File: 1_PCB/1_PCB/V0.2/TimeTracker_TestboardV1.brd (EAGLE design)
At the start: 105.1 x 80 mm, 47 parts, among them IC1 L78L33ABUTR, IC2 7805DT, IC3 PCF8574T_3,518, IC4 PCF8574T_3,518, U1 WS2812B, U2 WS2812B, U3 WS2812B, U4 WS2812B, U5 SMTM1225, Y1 FX135A-327

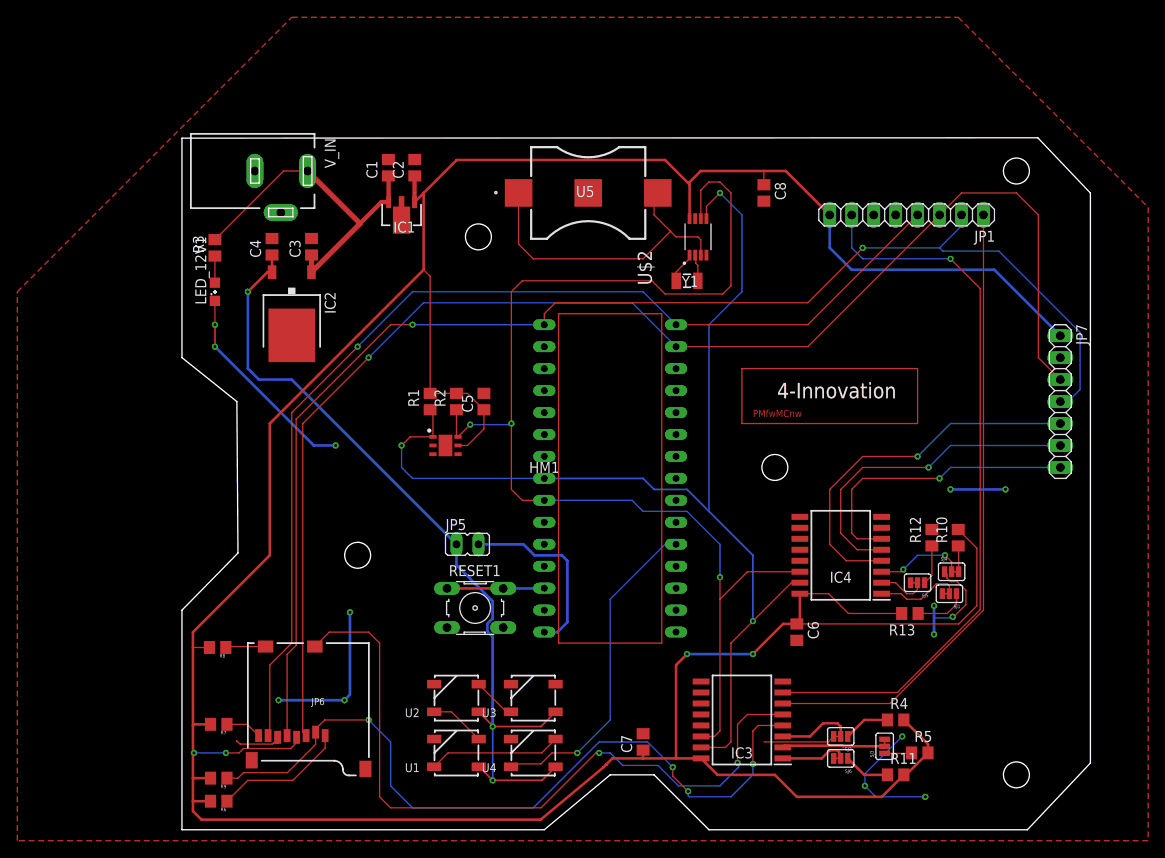
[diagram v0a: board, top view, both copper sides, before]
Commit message: Nicolas
PCB Update
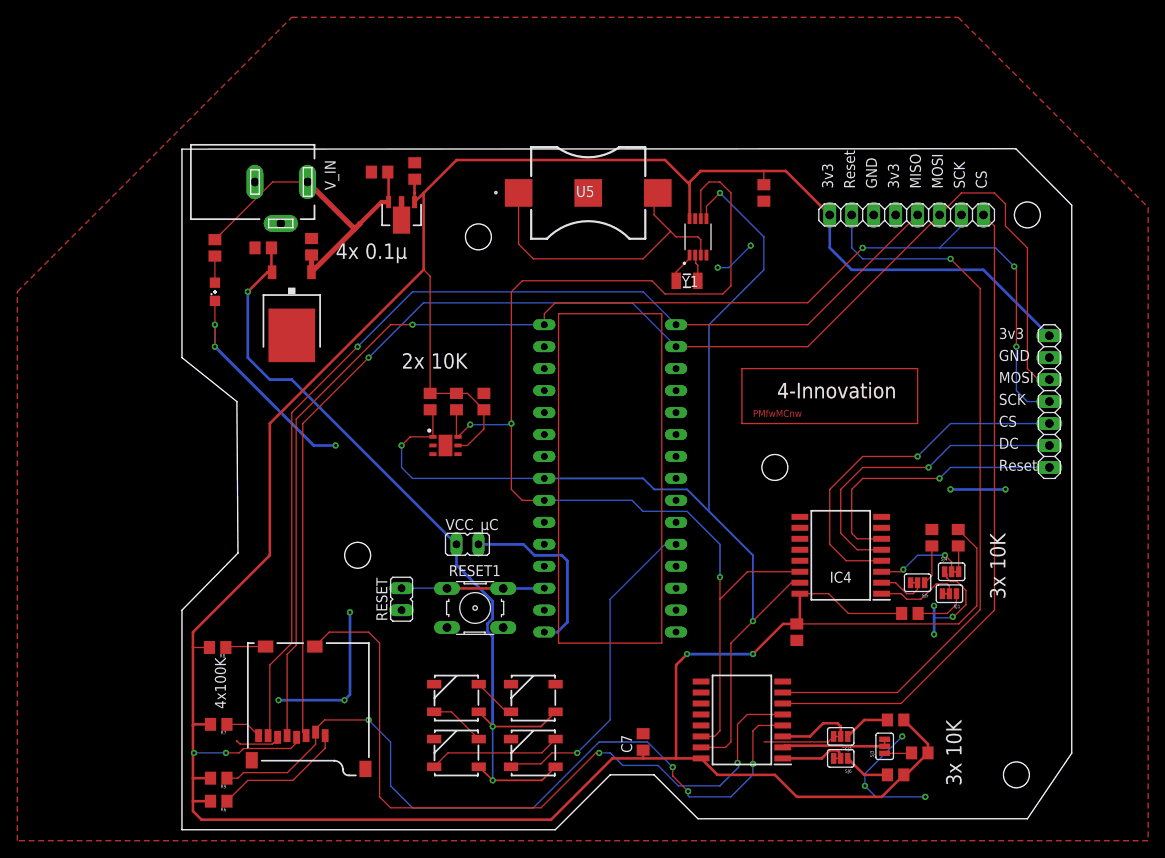
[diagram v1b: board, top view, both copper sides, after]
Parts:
- removed C1: (no value), rcl:C0805
- added 0.1µ: (no value), rcl:C0805
- added RESET: (no value), jumper:JP1
- C2, C6, C8: value (none) -> 0,1µ
- moved V_IN 1.27 mm to (8.89, 73.7)
- moved JP7 1.27 mm to (97.8, 48.3)
- moved C4 1.02 mm to (6.86, 66.0), turned to 180 degrees
- moved C2 0.38 mm to (24.4, 74.9)
- renumbered JP5 to VCC_µC
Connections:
- net GND: now also 0.1µ.2, RESET.1; no longer C1.2
- net GND1: now also RESET.2
- net N$1: now also 0.1µ.1; no longer C1.1
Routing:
- net GND1: track 11.3 -> 16.5 mm
- net GND: track 92.9 -> 97.7 mm, vias 14 -> 16
- net I2CSDA: track 131.4 -> 133.5 mm
- net RFID_CS: track 73.4 -> 75.2 mm
- net 3V3: track 401.3 -> 399.8 mm
- net SPISCK: track 155.1 -> 153.6 mm, vias 2 -> 4
- net SPIMOSI: track 157.8 -> 156.5 mm
- net DISPLAY_RESET: track 34.0 -> 32.7 mm
- net DISPLAY_DC: track 38.1 -> 36.8 mm
- net DISPLAY_CS: track 43.0 -> 41.7 mm
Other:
- board size 105.1 x 80 mm -> 102.9 x 78.8 mm
- board text added: "2x 10K"
- board text added: "3v3"
- board text added: "3x 10K"
- board text added: "4x 0.1µ"
- board text added: "4x100K"
- board text added: "CS"
- board text added: "DC"
- board text added: "GND"
- board text added: "MISO"
- board text added: "MOSI"
- board text added: "Reset"
- board text added: "SCK"
